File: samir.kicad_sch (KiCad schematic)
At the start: 0 parts

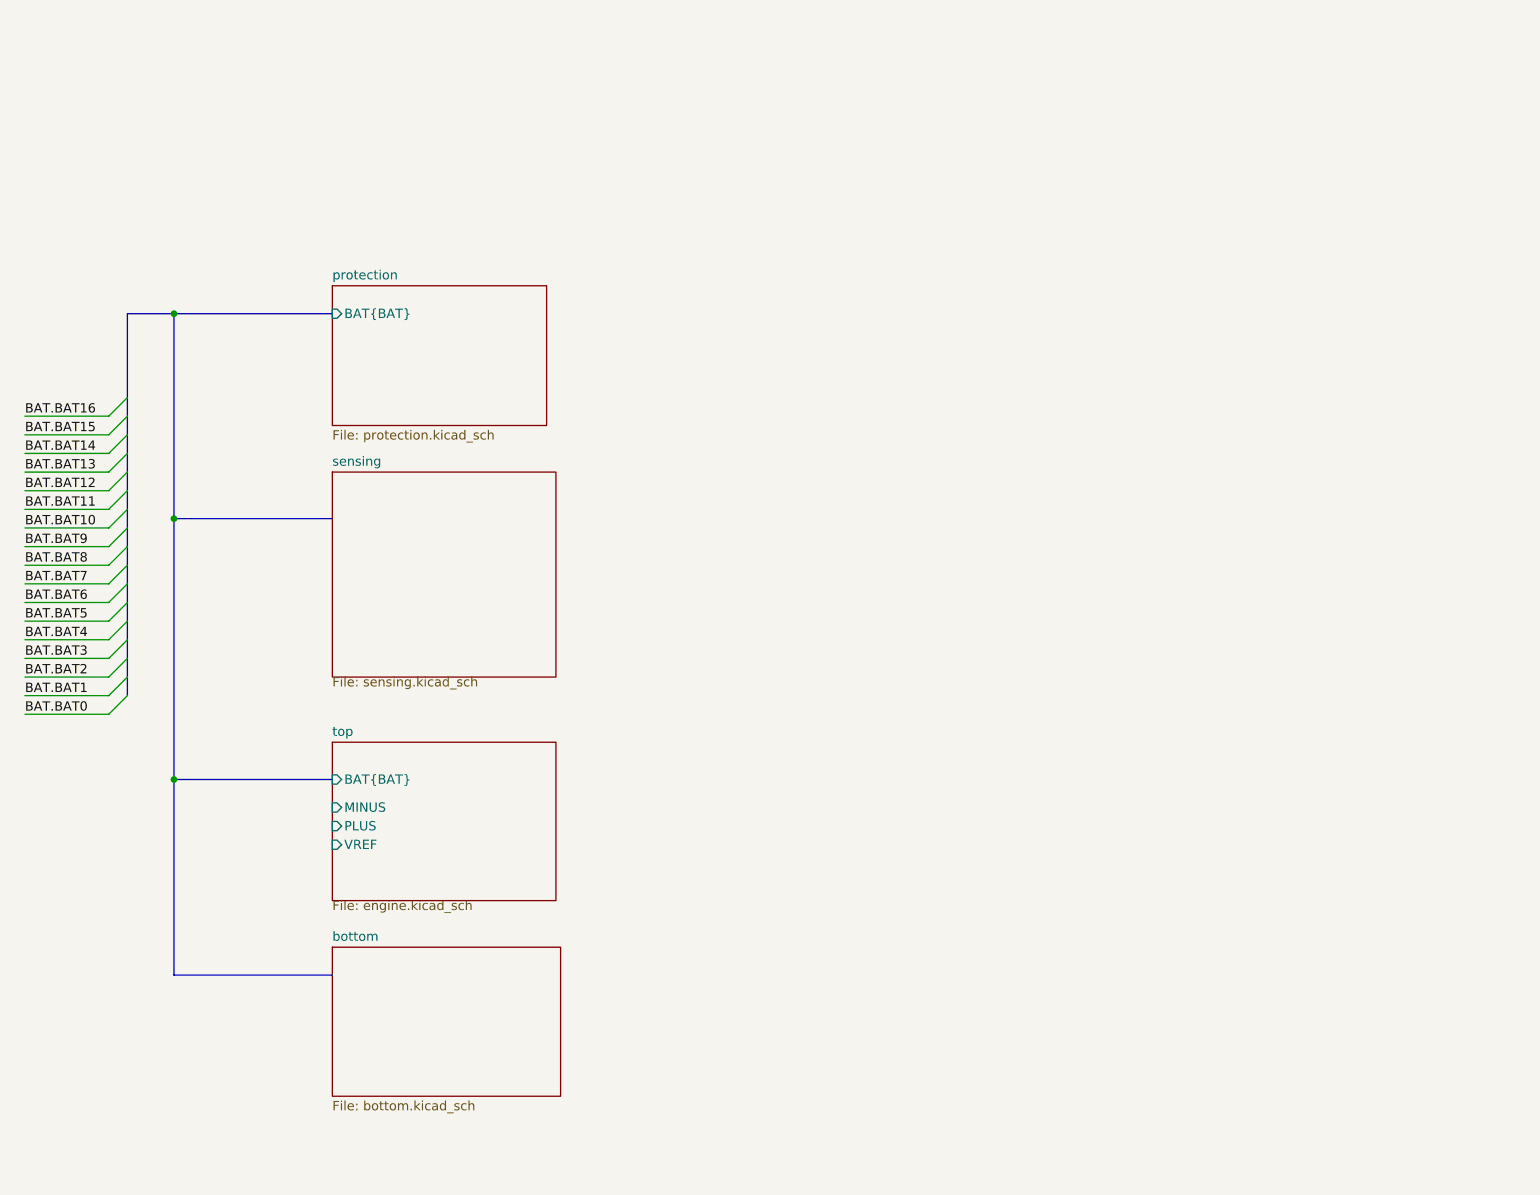
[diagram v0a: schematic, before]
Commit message: stuff
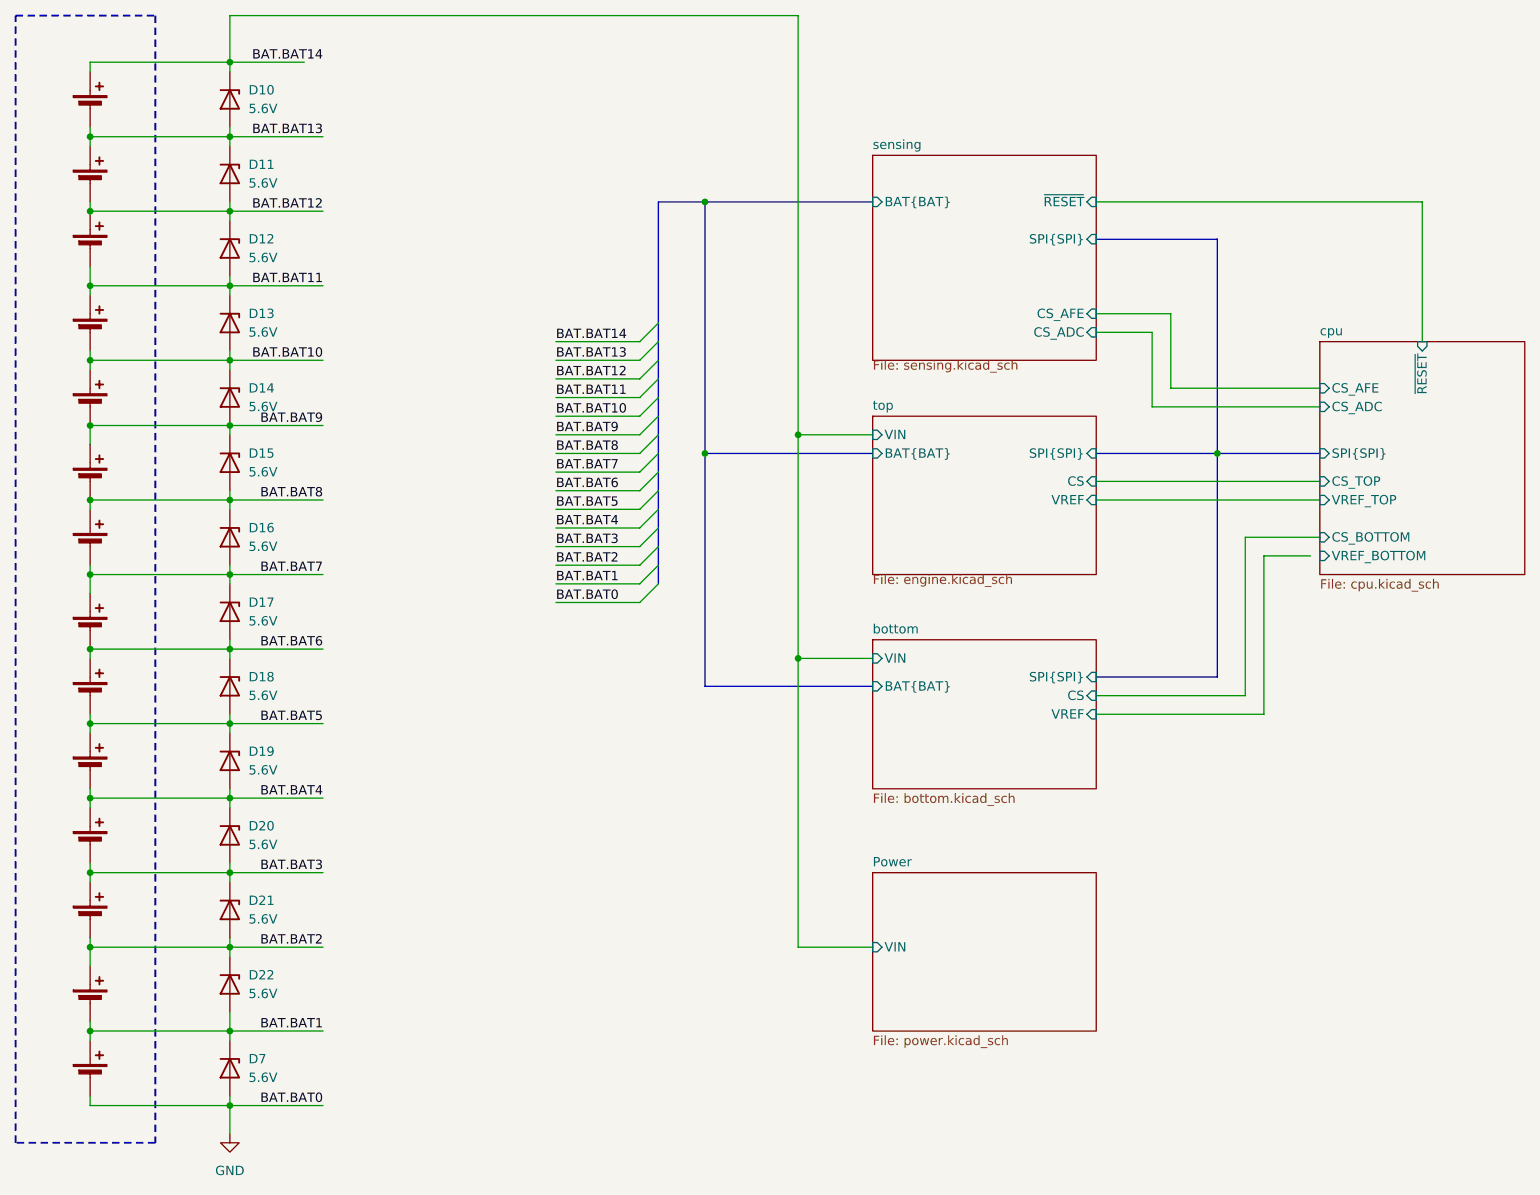
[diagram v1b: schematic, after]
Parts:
- added BT1, BT10, BT11, BT12, BT13, BT14, BT2, BT3, BT4, BT5, BT6, BT7, BT8, BT9: Battery_Cell, symbol Device:Battery_Cell
- added D10, D11, D12, D13, D14, D15, D16, D17, D18, D19, D20, D21, D22, D7: 5.6V, symbol Device:D_Zener
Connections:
- net BAT.BAT1: now also BT13.2 (-), BT14.1 (+), D22.2 (A), D7.1 (K)
- net BAT.BAT10: now also BT4.2 (-), BT5.1 (+), D13.2 (A), D14.1 (K)
- net BAT.BAT11: now also BT3.2 (-), BT4.1 (+), D12.2 (A), D13.1 (K)
- net BAT.BAT12: now also BT2.2 (-), BT3.1 (+), D11.2 (A), D12.1 (K)
- net BAT.BAT13: now also BT1.2 (-), BT2.1 (+), D10.2 (A), D11.1 (K)
- net BAT.BAT2: now also BT12.2 (-), BT13.1 (+), D21.2 (A), D22.1 (K)
- net BAT.BAT3: now also BT11.2 (-), BT12.1 (+), D20.2 (A), D21.1 (K)
- net BAT.BAT4: now also BT10.2 (-), BT11.1 (+), D19.2 (A), D20.1 (K)
- net BAT.BAT5: now also BT10.1 (+), BT9.2 (-), D18.2 (A), D19.1 (K)
- net BAT.BAT6: now also BT8.2 (-), BT9.1 (+), D17.2 (A), D18.1 (K)
- net BAT.BAT7: now also BT7.2 (-), BT8.1 (+), D16.2 (A), D17.1 (K)
- net BAT.BAT8: now also BT6.2 (-), BT7.1 (+), D15.2 (A), D16.1 (K)
- net BAT.BAT9: now also BT5.2 (-), BT6.1 (+), D14.2 (A), D15.1 (K)
- new net GND: BT14.2 (-), D7.2 (A)
- new net Power/VIN: BT1.1 (+), D10.1 (K)
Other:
- removed sheet protection
- added sheet Power (power.kicad_sch)
- added sheet cpu (cpu.kicad_sch)
- sheet bottom ports: added BAT{BAT}, CS, SPI{SPI}, VIN, VREF; removed none
- sheet sensing ports: added BAT{BAT}, CS_ADC, CS_AFE, SPI{SPI}, ~{RESET}; removed none
- sheet top ports: added CS, SPI{SPI}, VIN; removed MINUS, PLUS
